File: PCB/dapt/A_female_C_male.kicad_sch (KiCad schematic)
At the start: 4 parts

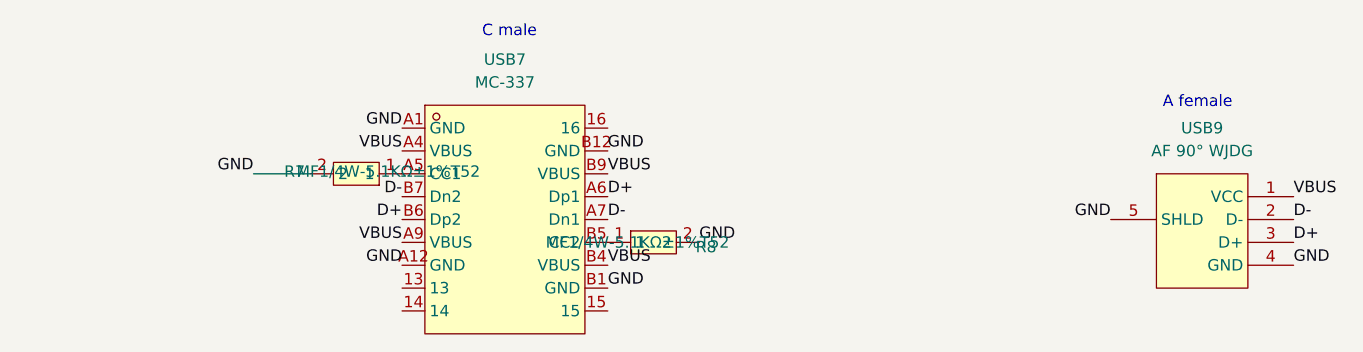
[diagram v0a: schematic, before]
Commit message: a
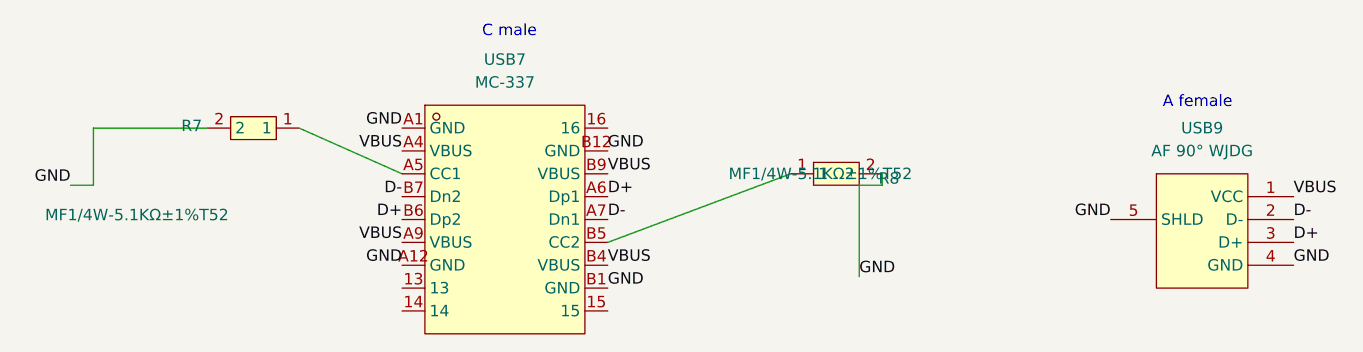
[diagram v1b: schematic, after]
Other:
- moved on the sheet: R7, R8
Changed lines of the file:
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@@
 	(wire
 		(pts
-			(xy 101.6 64.77) (xy 107.95 64.77)
+			(xy 106.68 59.69) (xy 118.11 64.77)
 		)
 		(stroke
@@
 		)
 	)
+	(wire
+		(pts
+			(xy 83.82 66.04) (xy 83.82 59.69)
+		)
+		(stroke
+			(width 0)
+			(type default)
+		)
+	)
+	(wire
+		(pts
+			(xy 161.29 64.77) (xy 140.97 72.39)
+		)
+		(stroke
+			(width 0)
+			(type default)
+		)
+	)
+	(wire
+		(pts
+			(xy 171.45 66.04) (xy 168.91 66.04)
+		)
+		(stroke
+			(width 0)
+			(type default)
+		)
+	)
+	(wire
+		(pts
+			(xy 83.82 59.69) (xy 96.52 59.69)
+		)
+		(stroke
+			(width 0)
+			(type default)
+		)
+	)
+	(wire
+		(pts
+			(xy 81.28 66.04) (xy 83.82 66.04)
+		)
+		(stroke
+			(width 0)
+			(type default)
+		)
+	)
+	(wire
+		(pts
+			(xy 171.45 66.04) (xy 171.45 64.77)
+		)
+		(stroke
+			(width 0)
+			(type default)
+		)
+	)
+	(wire
+		(pts
+			(xy 168.91 66.04) (xy 168.91 76.2)
+		)
+		(stroke
+			(width 0)
+			(type default)
+		)
+	)
 	(label "D+"
 		(at 217.17 72.39 0)
@@
 	)
 	(label "GND"
-		(at 101.6 64.77 180)
+		(at 81.28 66.04 180)
 		(effects
 			(font
@@
 	)
 	(label "GND"
-		(at 151.13 72.39 0)
+		(at 168.91 76.2 0)
 		(effects
 			(font
@@
 	(symbol
 		(lib_id "lcsc:MF1_4W-5.1KΩ±1%T52")
-		(at 146.05 72.39 0)
+		(at 166.37 64.77 0)
 		(unit 1)
 		(body_style 1)
@@
 		(dnp no)
 		(property "Reference" "R8"
-			(at 151.892 72.898 0)
+			(at 172.212 65.278 0)
 			(show_name no)
 			(do_not_autoplace no)
@@
 		)
 		(property "Value" "MF1/4W-5.1KΩ±1%T52"
-			(at 144.272 72.39 0)
+			(at 164.592 64.77 0)
 			(show_name no)
 			(do_not_autoplace no)
@@
 		)
 		(property "Footprint" "easyeda2kicad:RES-TH_BD2.3-L6.5-P10.50-D0.5"
-			(at 146.05 80.01 0)
+			(at 166.37 72.39 0)
 			(hide yes)
 			(show_name no)
@@
 		)
 		(property "Datasheet" "https://lcsc.com/product-detail/Metal-Film-Resistor-TH_Huaxing-Mechanical-Elec-MF1-4W-5-1KO-1-T52_C714010.html"
-			(at 146.05 82.55 0)
+			(at 166.37 74.93 0)
 			(hide yes)
 			(show_name no)
@@
 		)
 		(property "Description" ""
-			(at 146.05 72.39 0)
+			(at 166.37 64.77 0)
 			(hide yes)
 			(show_name no)
@@
 		)
 		(property "Manufacturer" "华星机电"
-			(at 146.05 85.09 0)
+			(at 166.37 77.47 0)
 			(hide yes)
 			(show_name no)
@@
 		)
 		(property "MPN" "MF1/4W-5.1KΩ±1%T52"
-			(at 146.05 87.63 0)
+			(at 166.37 80.01 0)
 			(hide yes)
 			(show_name no)
@@
 		)
 		(property "LCSC Part" "C714010"
-			(at 146.05 90.17 0)
+			(at 166.37 82.55 0)
 			(hide yes)
 			(show_name no)
@@
 	(symbol
 		(lib_id "lcsc:MF1_4W-5.1KΩ±1%T52")
-		(at 113.03 64.77 180)
+		(at 101.6 59.69 180)
 		(unit 1)
 		(body_style 1)
@@
 		(dnp no)
 		(property "Reference" "R7"
-			(at 106.172 64.516 0)
+			(at 94.742 59.436 0)
 			(show_name no)
 			(do_not_autoplace no)
@@
 		)
 		(property "Value" "MF1/4W-5.1KΩ±1%T52"
-			(at 116.586 64.516 0)
+			(at 88.646 69.342 0)
 			(show_name no)
 			(do_not_autoplace no)
@@
 		)
 		(property "Footprint" "easyeda2kicad:RES-TH_BD2.3-L6.5-P10.50-D0.5"
-			(at 113.03 57.15 0)
+			(at 101.6 52.07 0)
 			(hide yes)
 			(show_name no)
@@
 		)
 		(property "Datasheet" "https://lcsc.com/product-detail/Metal-Film-Resistor-TH_Huaxing-Mechanical-Elec-MF1-4W-5-1KO-1-T52_C714010.html"
-			(at 113.03 54.61 0)
+			(at 101.6 49.53 0)
 			(hide yes)
 			(show_name no)
@@
 		)
 		(property "Description" ""
-			(at 113.03 64.77 0)
+			(at 101.6 59.69 0)
 			(hide yes)
 			(show_name no)
@@
 		)
 		(property "Manufacturer" "华星机电"
-			(at 113.03 52.07 0)
+			(at 101.6 46.99 0)
 			(hide yes)
 			(show_name no)
@@
 		)
 		(property "MPN" "MF1/4W-5.1KΩ±1%T52"
-			(at 113.03 49.53 0)
+			(at 101.6 44.45 0)
 			(hide yes)
 			(show_name no)
@@
 		)
 		(property "LCSC Part" "C714010"
-			(at 113.03 46.99 0)
-			(hide yes)
-			(show_name no)
+			(at 101.6 41.91 0)
+			(hide yes)
+			(show_name no)
